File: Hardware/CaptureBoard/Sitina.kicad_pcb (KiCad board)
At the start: 2 copper layers, 67 x 39 mm, 211 parts, among them J100 Conn_01x30_MountingPin, Q1000 DMC3071LVT, Q1001 DMC3071LVT, Q1002 DMC3071LVT, Q1003 DMC3071LVT, Q1100 BC847BPN, U1 ADA4800, U10 LT1964-BYP, U11 LT1964-BYP, U1200 KAI-1100x, U2 ADA4800, U4 LT3472, U5 LT3472, U6 LT3472, U7 LT3023, U8 LT3023, U800 AD9990, U900 74LCX541BQX, U901 74LCX541BQX, U902 74LCX541BQX, U903 74LCX541BQX, Y800 30MHz

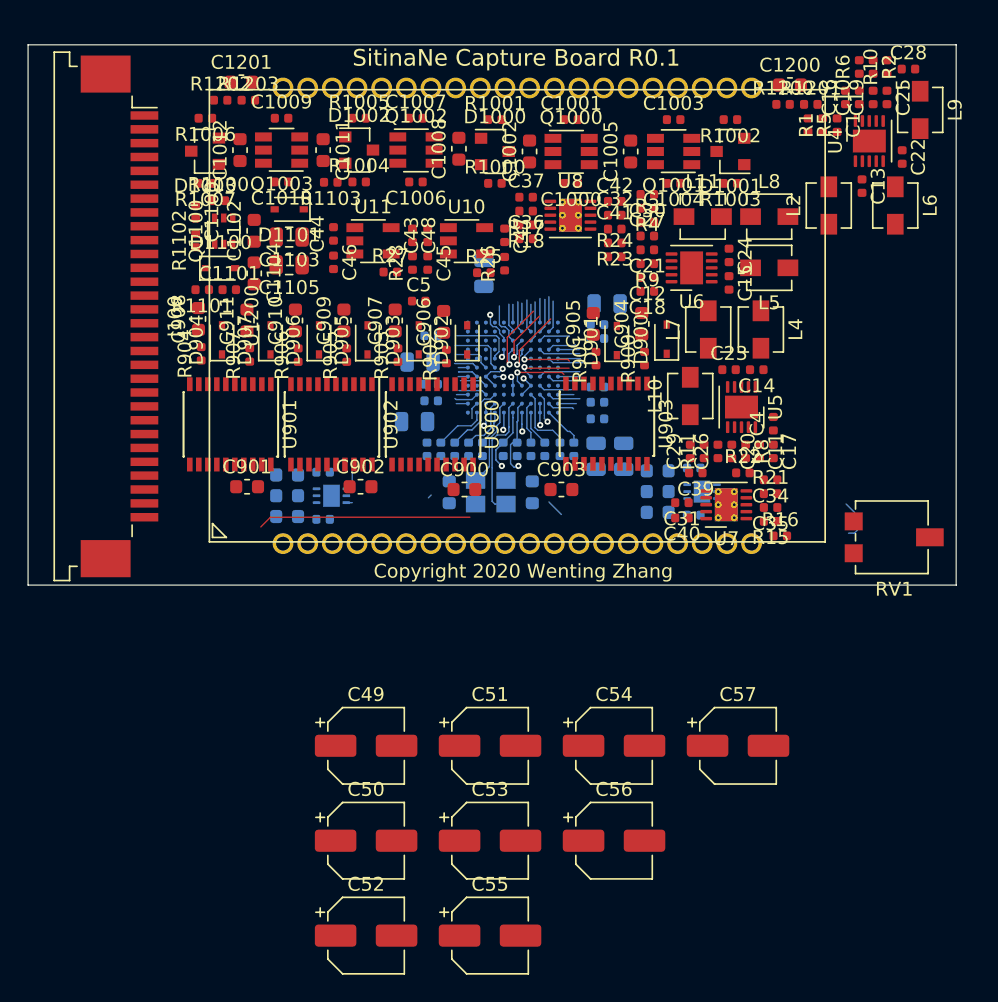
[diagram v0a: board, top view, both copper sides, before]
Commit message: pcb: wip
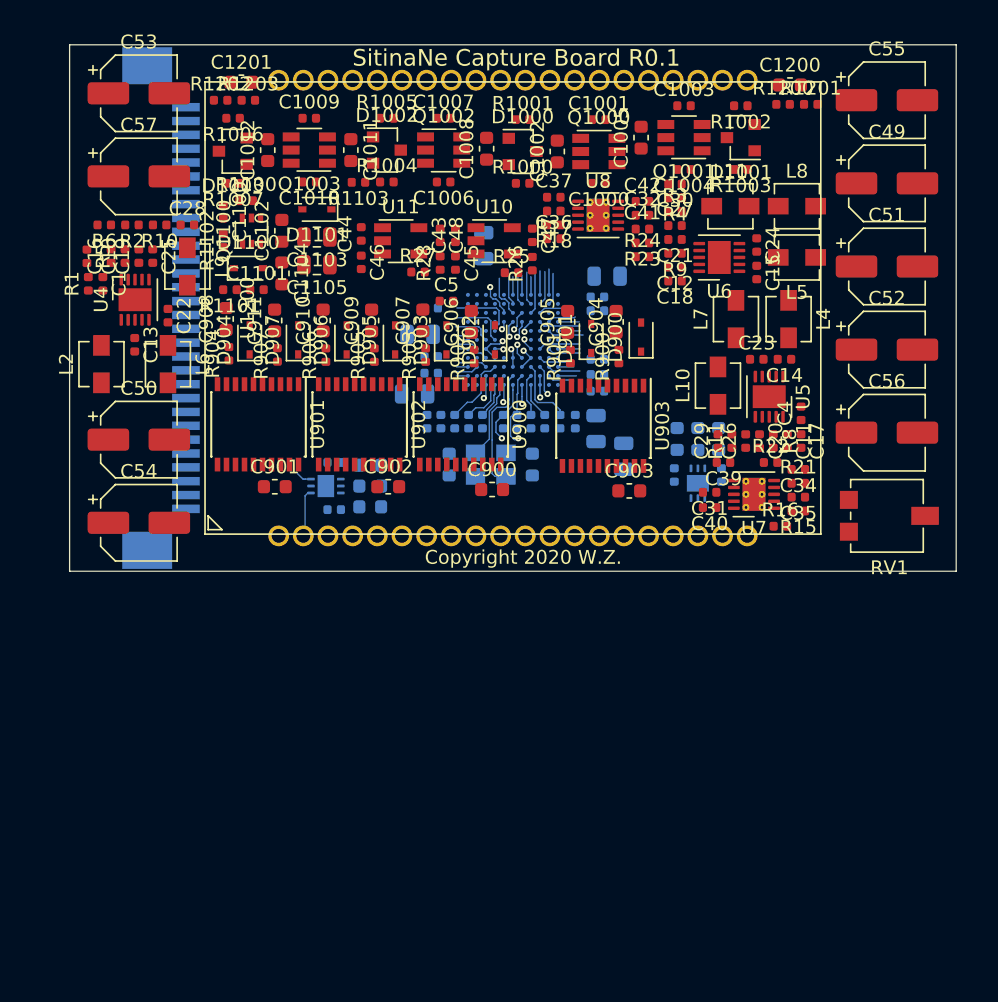
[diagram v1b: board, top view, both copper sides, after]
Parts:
- J100: moved to B.Cu
- moved C55 66.8 mm to (172.0, 86.0)
- moved C57 59.7 mm to (118.0, 91.5)
- moved C53 59.6 mm to (118.0, 85.5)
- moved C52 56.6 mm to (172.0, 104.0)
- moved R6 55.7 mm to (115.5, 95.0), turned to 180 degrees
- moved C49 55.3 mm to (172.0, 92.0)
- moved R2 54.7 mm to (117.5, 95.0), turned to 180 degrees
- moved C1 54.2 mm to (115.4, 99.2)
- moved C10 54.2 mm to (117.0, 97.2)
- moved C16 54.2 mm to (116.0, 97.2)
- moved C19 54.2 mm to (118.0, 97.2)
- moved C22 54.2 mm to (120.1, 101.5)
- moved C25 54.2 mm to (119.0, 97.2)
- moved R1 54.2 mm to (114.3, 99.2)
- moved U4 54.2 mm to (117.7, 100.4)
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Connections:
- U800 pad A10: Net-(C823-Pad1) -> Net-(C830-Pad1)
- U800 pad A2: Net-(C830-Pad1) -> Net-(C823-Pad1)
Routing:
- net Net-(C823-Pad2): track 17.1 -> 1.14 mm
- net /afe/CSI_D0: track 5.90 -> 1.21 mm
- net /afe/CSI_D7: track 5.52 -> 1.23 mm
- net Net-(C830-Pad1): track 3.82 -> 0.00 mm
- net /afe/CSI_D6: track 5.14 -> 1.43 mm
- net /afe/AFE_SL: track 4.67 -> 1.26 mm
- net /afe/AFE_RST: track 4.20 -> 0.90 mm
- net /afe/AFE_SCK: track 4.13 -> 0.88 mm
- net Net-(C823-Pad1): track 3.00 -> 0.00 mm
- net /afe/CCDIN_B: track 2.94 -> 0.00 mm
- net /afe/CCDIN_A: track 1.71 -> 3.46 mm
- net Net-(C830-Pad2): track 1.57 -> 0.00 mm
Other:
- board size 67 x 39 mm -> 64 x 38 mm
- board text added: "Copyright 2020 W.Z."
- board text removed: "Copyright 2020 Wenting Zhang"
